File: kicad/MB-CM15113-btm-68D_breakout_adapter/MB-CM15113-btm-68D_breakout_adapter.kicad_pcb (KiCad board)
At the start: 2 copper layers, 31.7 x 43.3 mm, 4 parts, among them P1 CONN_01X16, P2 CONN_01X05, P3 CONN_01X16, U1 MB-CM15113

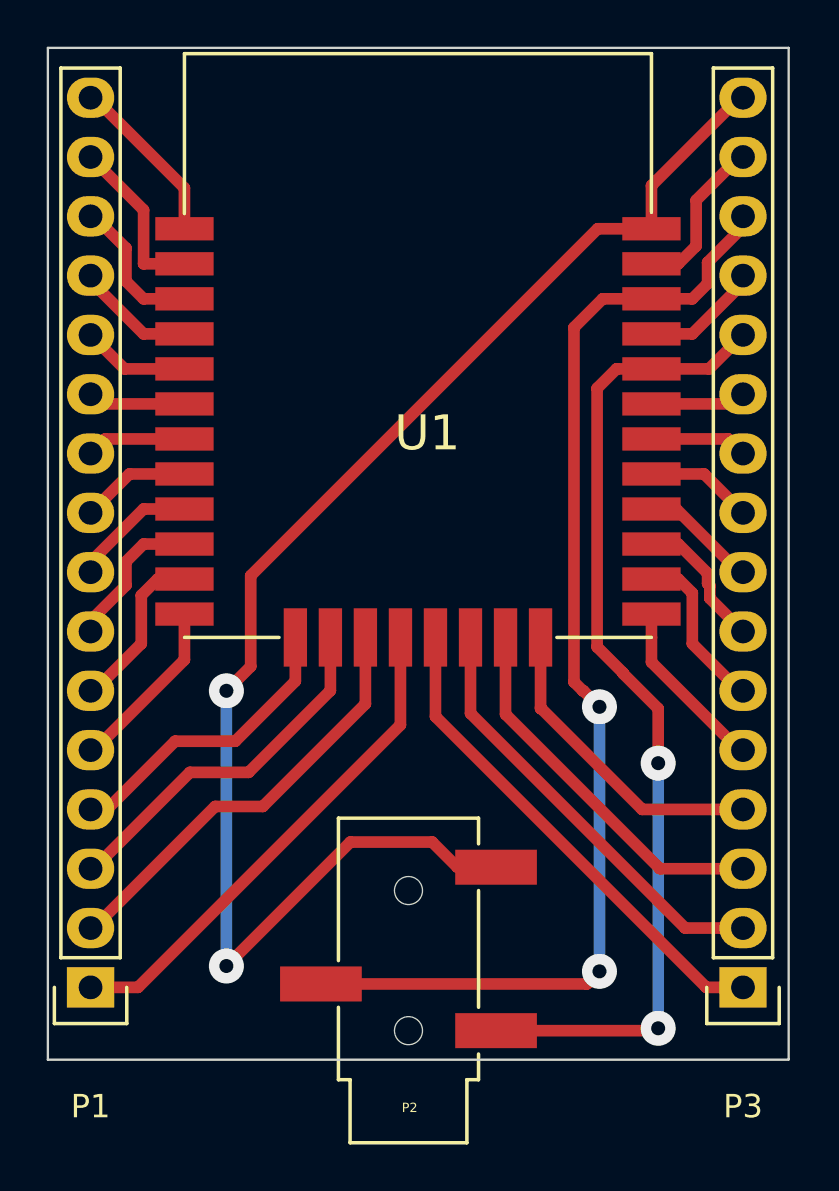
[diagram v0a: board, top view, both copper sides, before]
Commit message: update
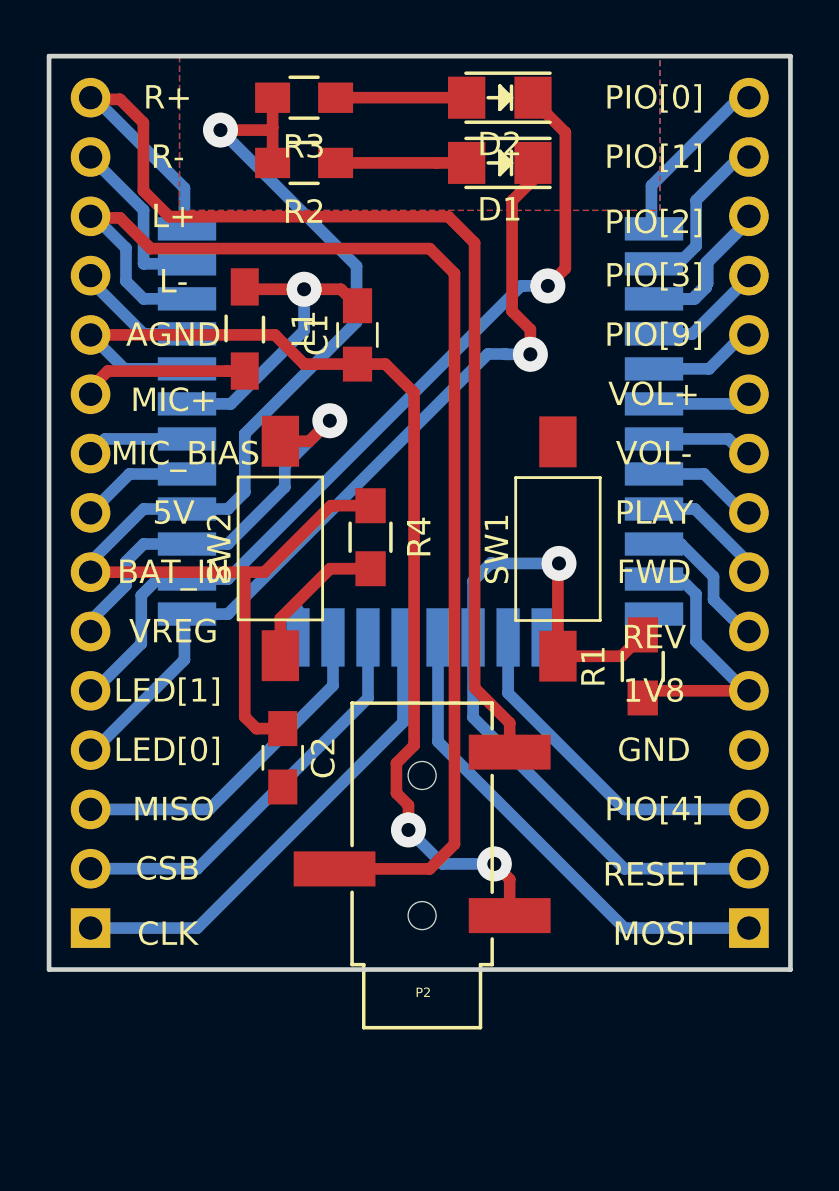
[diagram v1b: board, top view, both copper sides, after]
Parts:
- added C1: 15pF, Capacitors_SMD:C_0805_HandSoldering, F.Cu at (156.2, 97.8)
- added C2: 100n, Capacitors_SMD:C_0805_HandSoldering, F.Cu at (153.0, 115.9)
- added D1: D, LEDs.pretty:LED-1206, F.Cu at (162.3, 90.4)
- added D2: D, LEDs.pretty:LED-1206, F.Cu at (162.3, 87.6)
- added L1: 15nH, Choke_SMD:Choke_SMD_1206_Standard, F.Cu at (151.4, 97.5)
- added R1: 10k, Resistors_SMD.pretty:R_0805_HandSoldering, F.Cu at (168.4, 112.0)
- added R2: 470, Resistors_SMD.pretty:R_0805_HandSoldering, F.Cu at (153.9, 90.4)
- added R3: 470, Resistors_SMD.pretty:R_0805_HandSoldering, F.Cu at (153.9, 87.6)
- added R4: 10k, Resistors_SMD.pretty:R_0805_HandSoldering, F.Cu at (156.8, 106.5)
- added SW1: RESET, Buttons_Switches_SMD:SW_SPST_FSMSM, F.Cu at (164.8, 107.0)
- added SW2: ON/OFF, Buttons_Switches_SMD:SW_SPST_FSMSM, F.Cu at (152.9, 106.9)
- P1, P3: value CONN_01X16 -> CONN_01X15; footprint Pin_Headers:Pin_Header_Straight_1x16 -> Pin_Headers:Pin_Header_Straight_1x15_Pitch2.54mm; moved to B.Cu
- U1: moved to B.Cu
- moved P1 28.3 mm to (173.0, 123.2), turned to 0 degrees
- moved P3 28.1 mm to (144.8, 123.2), turned to 0 degrees
- moved U1 20.1 mm to (168.9, 110.7), turned to 180 degrees
- moved P2 4.96 mm to (159.0, 122.7)
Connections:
- P1 pad 4: Net-(P1-Pad4) -> GND
- P2 pad 1: Net-(P2-Pad1) -> Net-(C1-Pad1)
- P3 pad 10: Net-(P3-Pad10) -> Net-(L1-Pad2)
- P3 pad 11: Net-(P3-Pad11) -> Net-(C1-Pad1)
- P3 pad 12: Net-(P2-Pad1) -> Net-(P3-Pad12)
- P3 pad 13: Net-(P3-Pad13) -> Net-(P2-Pad2)
- P3 pad 14: Net-(P2-Pad2) -> Net-(P3-Pad14)
- P3 pad 15: Net-(P3-Pad15) -> Net-(P2-Pad5)
- P3 pad 4: Net-(P3-Pad4) -> Net-(D1-Pad1)
- P3 pad 5: Net-(P3-Pad5) -> Net-(D2-Pad1)
- P3 pad 7: Net-(P3-Pad7) -> Net-(C2-Pad1)
- U1 pad 1: Net-(P1-Pad16) -> Net-(P1-Pad15)
- U1 pad 10: Net-(P1-Pad7) -> Net-(P1-Pad6)
- U1 pad 11: Net-(P1-Pad6) -> Net-(P1-Pad5)
- U1 pad 12: Net-(P1-Pad5) -> GND
- U1 pad 13: Net-(P1-Pad4) -> GND
- U1 pad 2: Net-(P1-Pad15) -> Net-(P1-Pad14)
- U1 pad 20: Net-(P3-Pad4) -> GND
- U1 pad 21: Net-(P3-Pad5) -> Net-(D1-Pad1)
- U1 pad 22: Net-(P3-Pad6) -> Net-(D2-Pad1)
- U1 pad 23: Net-(P3-Pad7) -> Net-(P3-Pad6)
- U1 pad 24: Net-(P3-Pad8) -> Net-(C2-Pad1)
- U1 pad 25: Net-(P3-Pad9) -> Net-(P3-Pad8)
- U1 pad 26: Net-(P3-Pad10) -> Net-(P3-Pad9)
- U1 pad 27: Net-(P3-Pad11) -> Net-(C1-Pad2)
- U1 pad 28: Net-(P2-Pad1) -> Net-(C1-Pad1)
- U1 pad 29: Net-(P3-Pad13) -> Net-(P3-Pad12)
- U1 pad 3: Net-(P1-Pad14) -> Net-(P1-Pad13)
- U1 pad 31: Net-(P3-Pad15) -> Net-(P3-Pad14)
- U1 pad 4: Net-(P1-Pad13) -> Net-(P1-Pad12)
- U1 pad 5: Net-(P1-Pad12) -> Net-(P1-Pad11)
- U1 pad 6: Net-(P1-Pad11) -> Net-(P1-Pad10)
- U1 pad 7: Net-(P1-Pad10) -> Net-(P1-Pad9)
- U1 pad 8: Net-(P1-Pad9) -> Net-(P1-Pad8)
- U1 pad 9: Net-(P1-Pad8) -> Net-(P1-Pad7)
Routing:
- net Net-(C2-Pad1): track 0.00 -> 54.3 mm, vias 0 -> 1
- net Net-(C1-Pad1): track 0.00 -> 45.8 mm, vias 0 -> 2
- net Net-(P2-Pad1): track 42.7 -> 0.00 mm, vias 2 -> 0
- net Net-(D2-Pad1): track 0.00 -> 37.5 mm, vias 0 -> 1
- net Net-(D1-Pad1): track 0.00 -> 35.8 mm, vias 0 -> 1
- net Net-(P1-Pad2): track 18.7 -> 32.4 mm, vias 0 -> 1
- net Net-(P3-Pad4): track 13.5 -> 0.00 mm
- net Net-(C1-Pad2): track 0.00 -> 13.2 mm, vias 0 -> 1
- net Net-(P1-Pad4): track 13.1 -> 0.00 mm
- net Net-(P2-Pad5): track 62.0 -> 50.8 mm, vias 2 -> 0
- net Net-(P3-Pad6): track 7.17 -> 17.8 mm, vias 0 -> 1
- net Net-(P3-Pad5): track 7.54 -> 0.00 mm
- net Net-(P1-Pad16): track 7.37 -> 0.00 mm
- net Net-(L1-Pad2): track 0.00 -> 7.27 mm
- net Net-(P3-Pad14): track 0.00 -> 7.26 mm
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- added copper zone on B.Cu, net GND
- added copper zone on F.Cu, net GND
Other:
- board size 31.7 x 43.3 mm -> 31.8 x 39.1 mm
- board text added: "1V8"
- board text added: "5V"
- board text added: "AGND"
- board text added: "BAT_IN"
- board text added: "CLK"
- board text added: "CSB"
- board text added: "FWD"
- board text added: "GND"
- board text added: "L+"
- board text added: "L-"
- board text added: "LED[0]"
- board text added: "LED[1]"
- board text added: "MIC+"
- board text added: "MIC_BIAS"
- board text added: "MISO"
- board text added: "MOSI"
- board text added: "PIO[0]"
- board text added: "PIO[1]"
- board text added: "PIO[2]"
- board text added: "PIO[3]"
- board text added: "PIO[4]"
- board text added: "PIO[9]"
- board text added: "PLAY"
- board text added: "R+"
- board text added: "R-"
- board text added: "RESET"
- board text added: "REV"
- board text added: "VOL+"
- board text added: "VOL-"
- board text added: "VREG"
